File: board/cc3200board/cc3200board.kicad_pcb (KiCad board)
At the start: 4 copper layers, 40.4 x 30.8 mm, 44 parts, among them P1 PROG, P3 CONN_JTAG, U1 CC3200R1M2RGCR, U2 N25Q128A13ESE40E, X1 32.768kH, X2 ABM3B-40.000MHZ-10-1-U-T

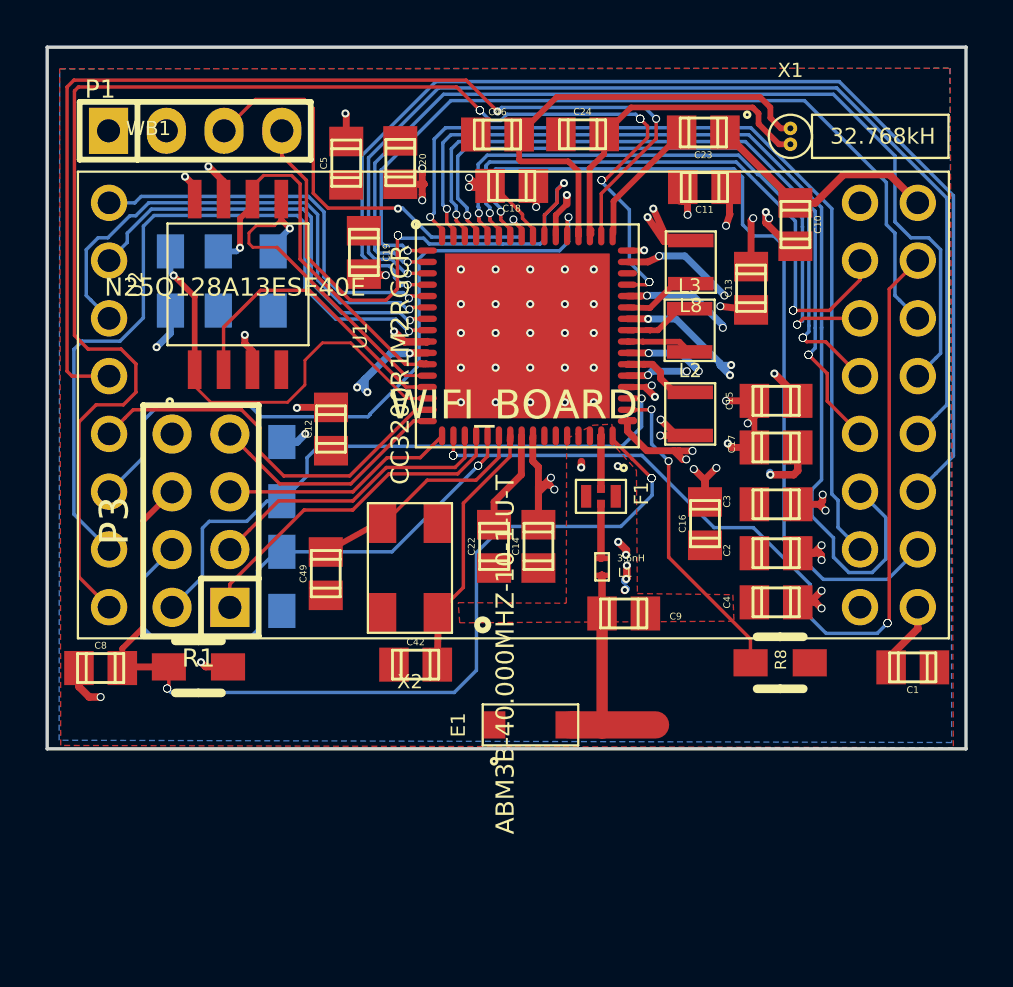
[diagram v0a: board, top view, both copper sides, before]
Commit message: Rev 1.0 of CC3200board
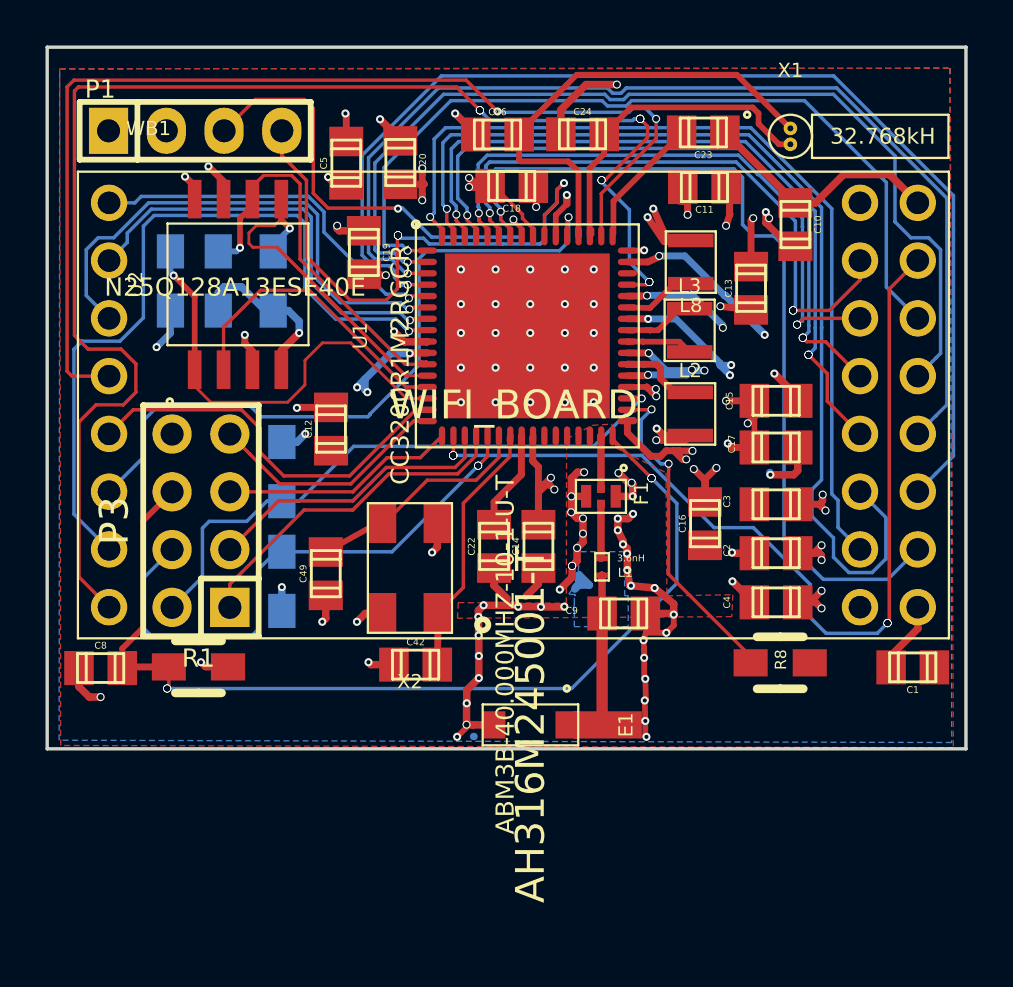
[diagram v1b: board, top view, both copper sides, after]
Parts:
- turned C9 to 180 degrees
- turned E1 to 270 degrees
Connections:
- C9 pad 1: GND -> /FEED
- E1 pad 1: GND -> /FEED
- L1 pad 2: GND -> /FEED
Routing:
- net GND: track 89.5 -> 143.7 mm, vias 39 -> 84
- net /FEED: track 0.00 -> 6.69 mm
- net 3V3: track 50.1 -> 53.1 mm
- net (no net): track 0.00 -> 1.97 mm
- net /cc3200-io/SOP0: track 28.3 -> 27.1 mm
- net /cc3200-io/GPIO14: track 17.7 -> 16.5 mm
- net /cc3200-io/nRESET: track 45.2 -> 45.9 mm
- net Net-(C46-Pad1): track 21.4 -> 22.0 mm
- net Net-(R8-Pad1): track 13.7 -> 14.3 mm
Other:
- net class 50OHM: clearance 0.127 -> 0
- net class FEED added: clearance 0, trace_width 0.5, via_dia 0.3556, via_drill 0.254
